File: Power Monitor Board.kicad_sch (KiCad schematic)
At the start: 43 parts, among them J1 Conn_01x02_Pin, J10 Conn_01x02_Pin, J11 Conn_01x02_Pin, J2 Conn_01x02_Pin, J5 Conn_01x02_Pin, J6 Conn_01x02_Pin, J7 Conn_01x02_Pin, J8 Conn_01x02_Pin, J9 Conn_01x02_Pin, U1 ACS711xLCTR-25AB, U2 ACS711xLCTR-25AB, U3 ACS711xLCTR-25AB, U4 ACS711xLCTR-25AB, U5 ACS711xLCTR-25AB, U6 ACS711xLCTR-25AB, U7 ACS711xLCTR-25AB, U8 ACS711xLCTR-25AB

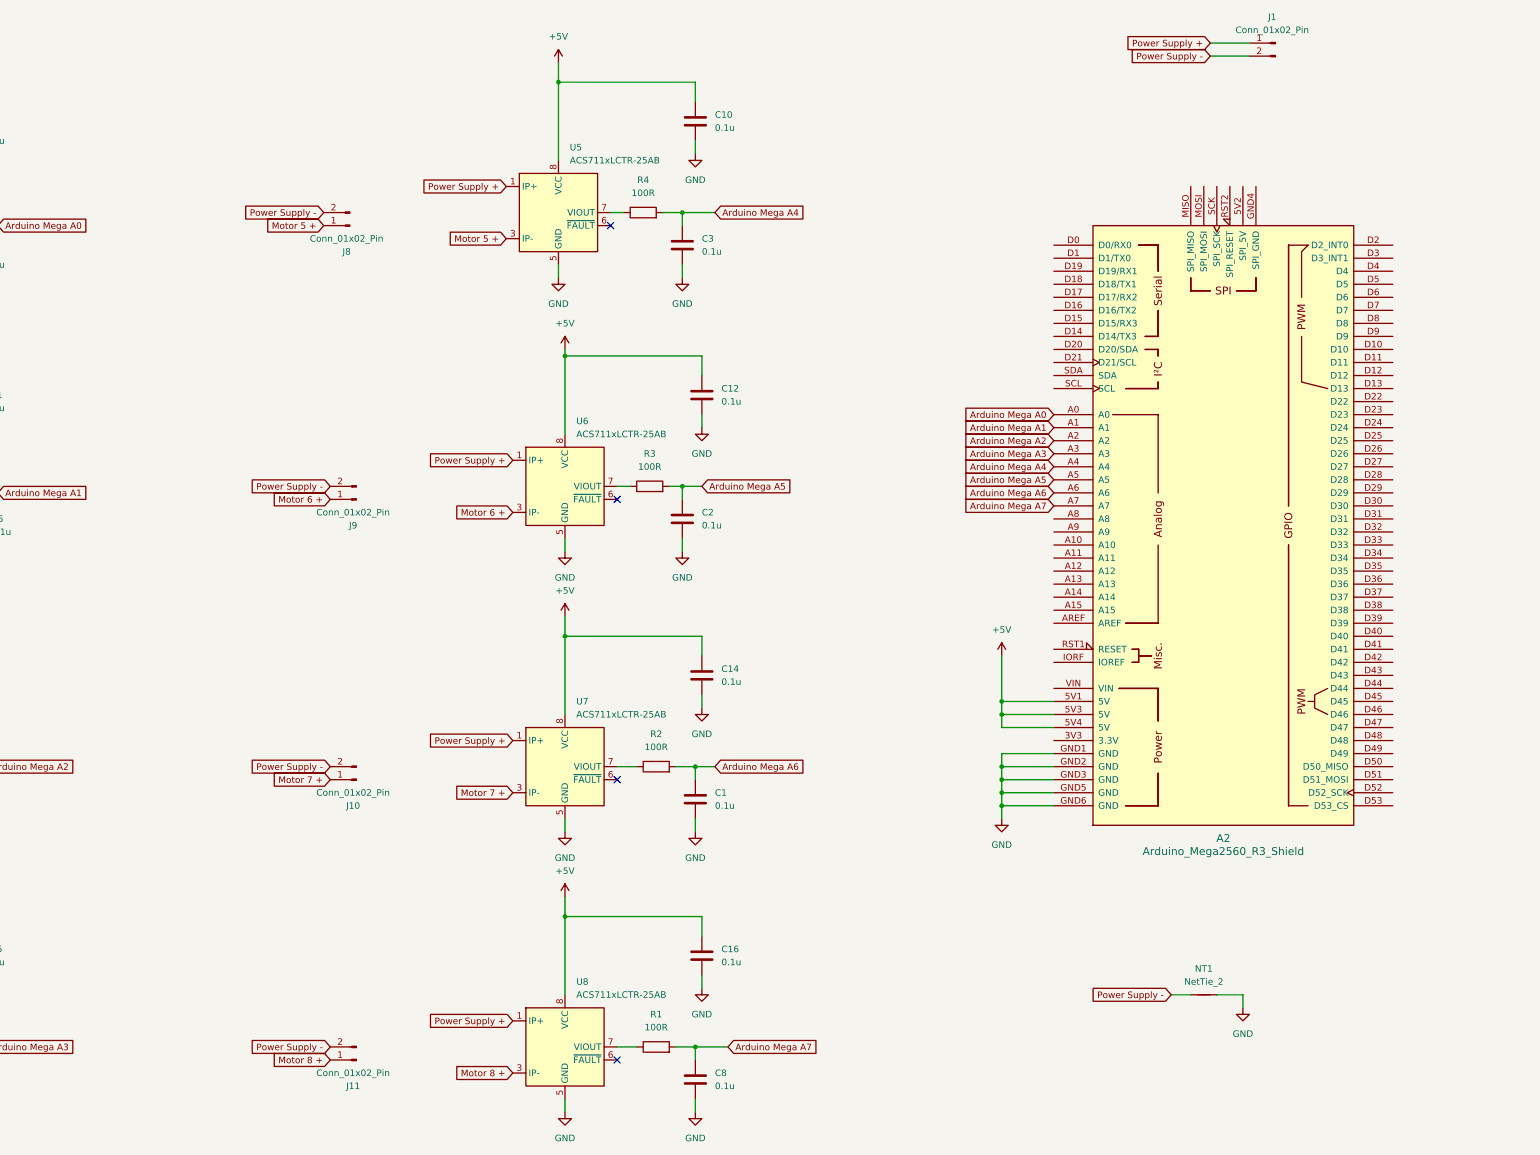
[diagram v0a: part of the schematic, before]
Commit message: Add files via upload
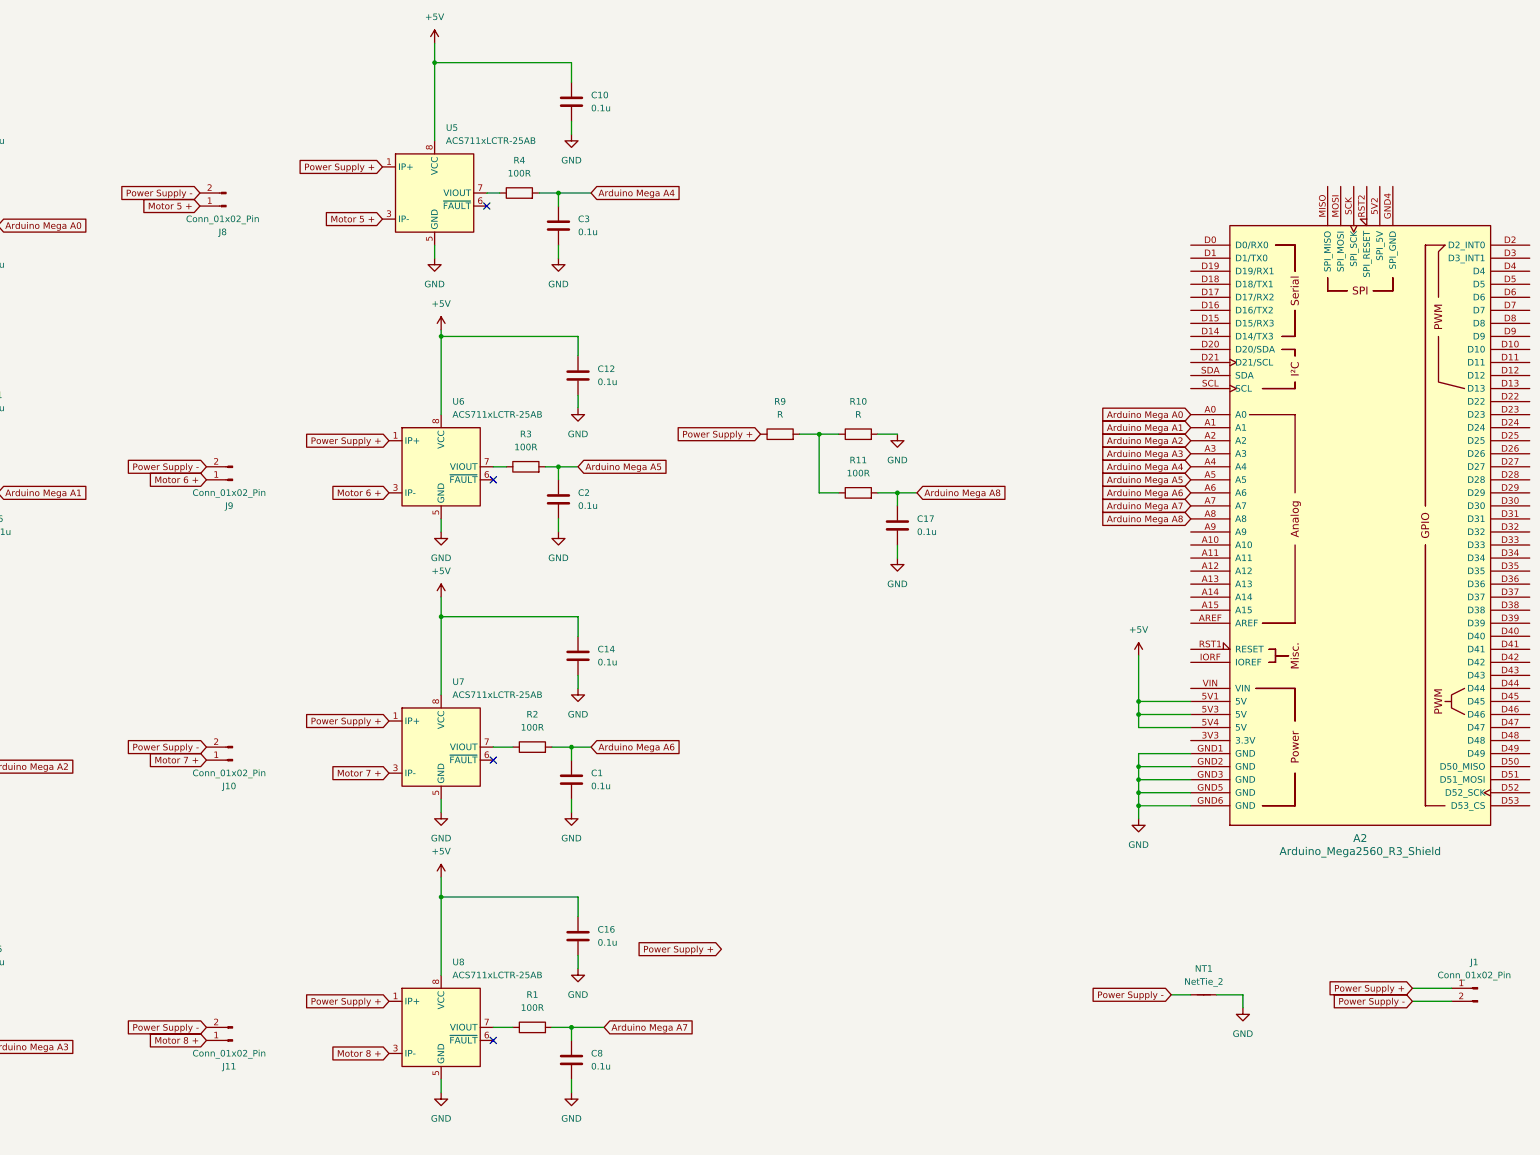
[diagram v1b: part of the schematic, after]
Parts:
- added C17: 0.1u, Capacitor_SMD:C_0603_1608Metric, symbol Device:C
- added R10, R9: R, Resistor_THT:R_Axial_DIN0309_L9.0mm_D3.2mm_P12.70mm_Horizontal, symbol Device:R
- added R11: 100R, Resistor_SMD:R_0603_1608Metric, symbol Device:R
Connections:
- net GND: now also C17.2, R10.2
- net Power Supply +: now also R9.1
- net Arduino Mega A8: now reaches A2.A8
- net Arduino Mega A8: now also C17.1, R11.2
- new net: R10.1, R11.1, R9.2
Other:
- moved on the sheet: A2, C1, C10, C12, C14, C16, C2, C3, C8, J1, J10, J11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
